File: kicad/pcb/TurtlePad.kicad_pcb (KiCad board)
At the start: 2 copper layers, 108 x 40 mm, 23 parts, among them SW1 SW_Push, U1 ProMicro

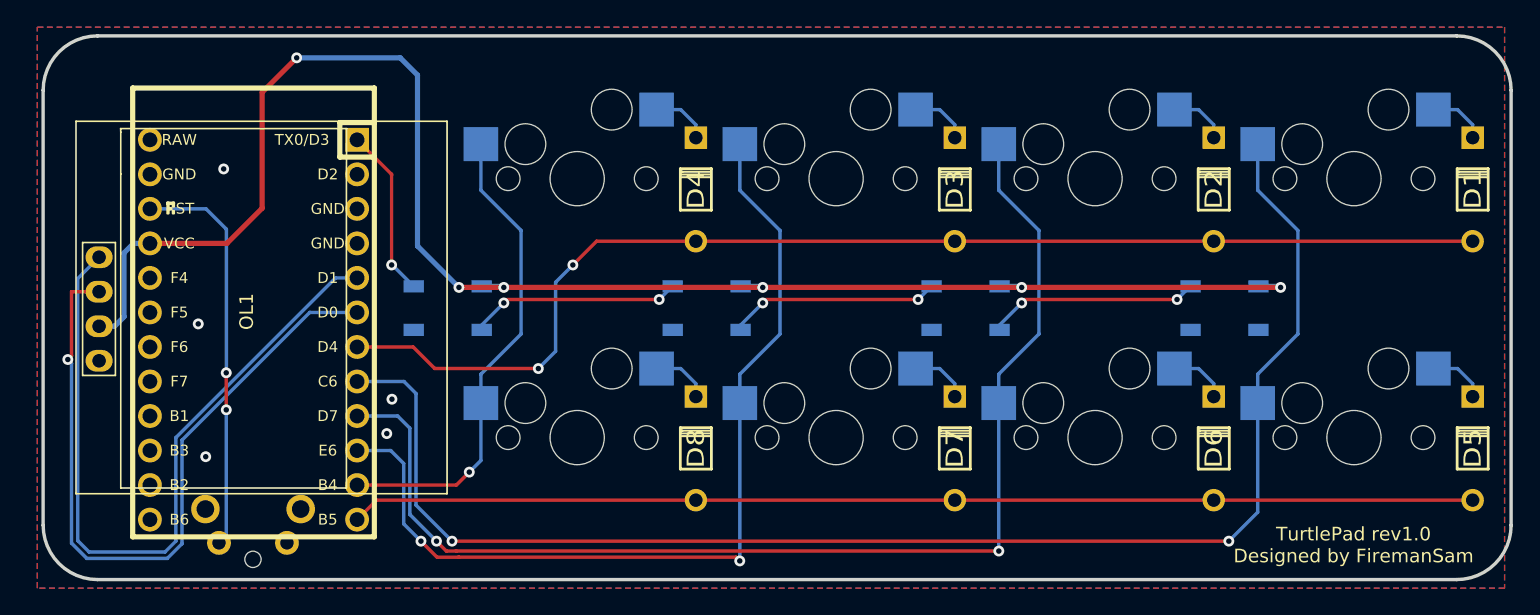
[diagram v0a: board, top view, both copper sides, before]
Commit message: plates and prod files
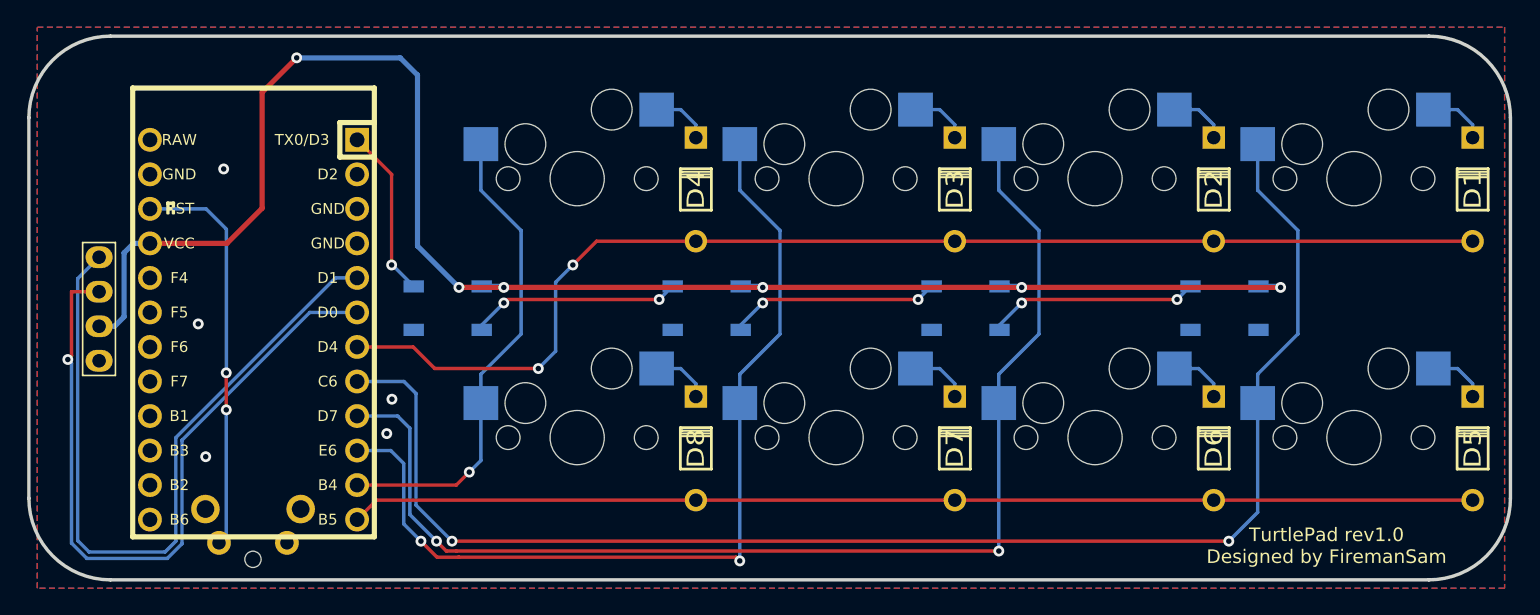
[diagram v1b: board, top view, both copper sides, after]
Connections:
- RGB4 pad 2: Net-(RGB4-Pad2) -> unconnected-(RGB4-Pad2)
- U1 pad 13: Net-(U1-Pad13) -> unconnected-(U1-Pad13)
- U1 pad 14: Net-(U1-Pad14) -> unconnected-(U1-Pad14)
- U1 pad 15: Net-(U1-Pad15) -> unconnected-(U1-Pad15)
- U1 pad 16: Net-(U1-Pad16) -> unconnected-(U1-Pad16)
- U1 pad 17: Net-(U1-Pad17) -> unconnected-(U1-Pad17)
- U1 pad 18: Net-(U1-Pad18) -> unconnected-(U1-Pad18)
- U1 pad 19: Net-(U1-Pad19) -> unconnected-(U1-Pad19)
- U1 pad 2: Net-(U1-Pad2) -> unconnected-(U1-Pad2)
- U1 pad 20: Net-(U1-Pad20) -> unconnected-(U1-Pad20)
- U1 pad 24: Net-(U1-Pad24) -> unconnected-(U1-Pad24)
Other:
- board size 108 x 40 mm -> 109 x 40 mm
